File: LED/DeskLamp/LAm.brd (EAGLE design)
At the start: 34.3 x 27.3 mm, 19 parts, among them IC1 INA168, IC3 LD2985BM50R, U1 TSV621ILT

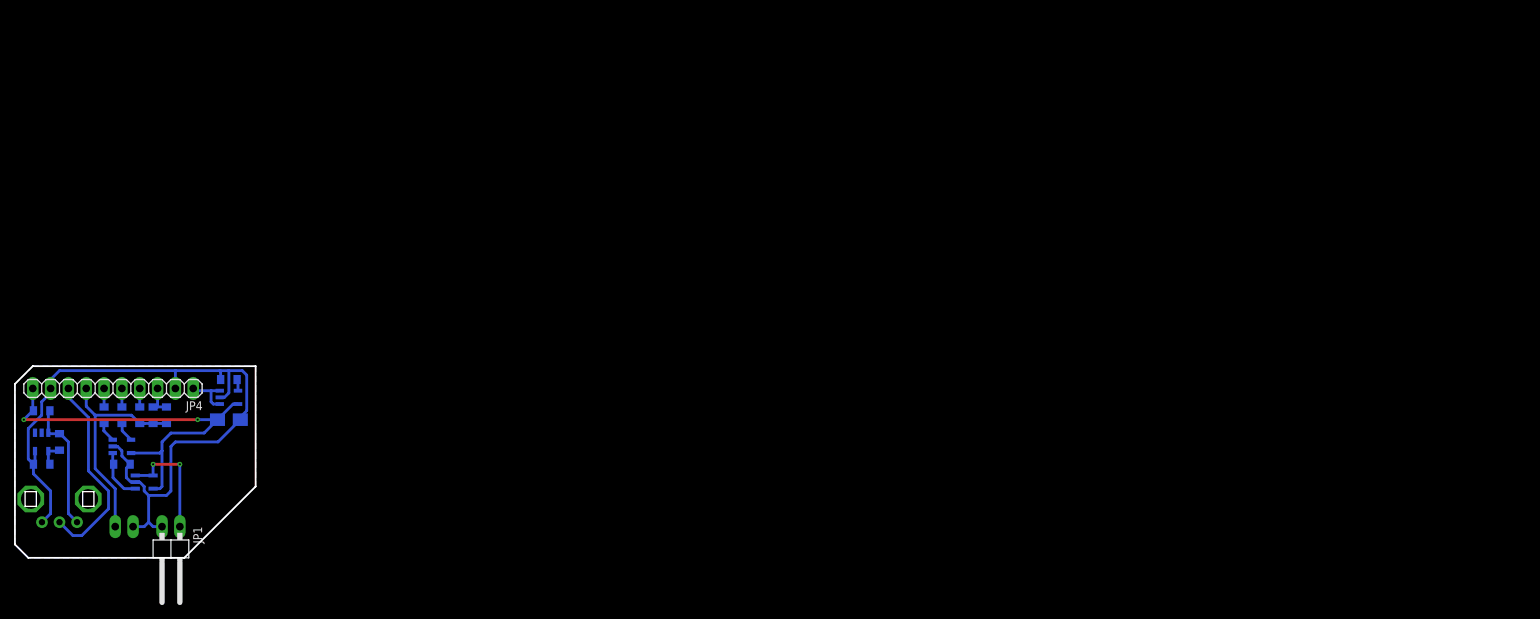
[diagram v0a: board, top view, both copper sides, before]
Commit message: DeskLamp
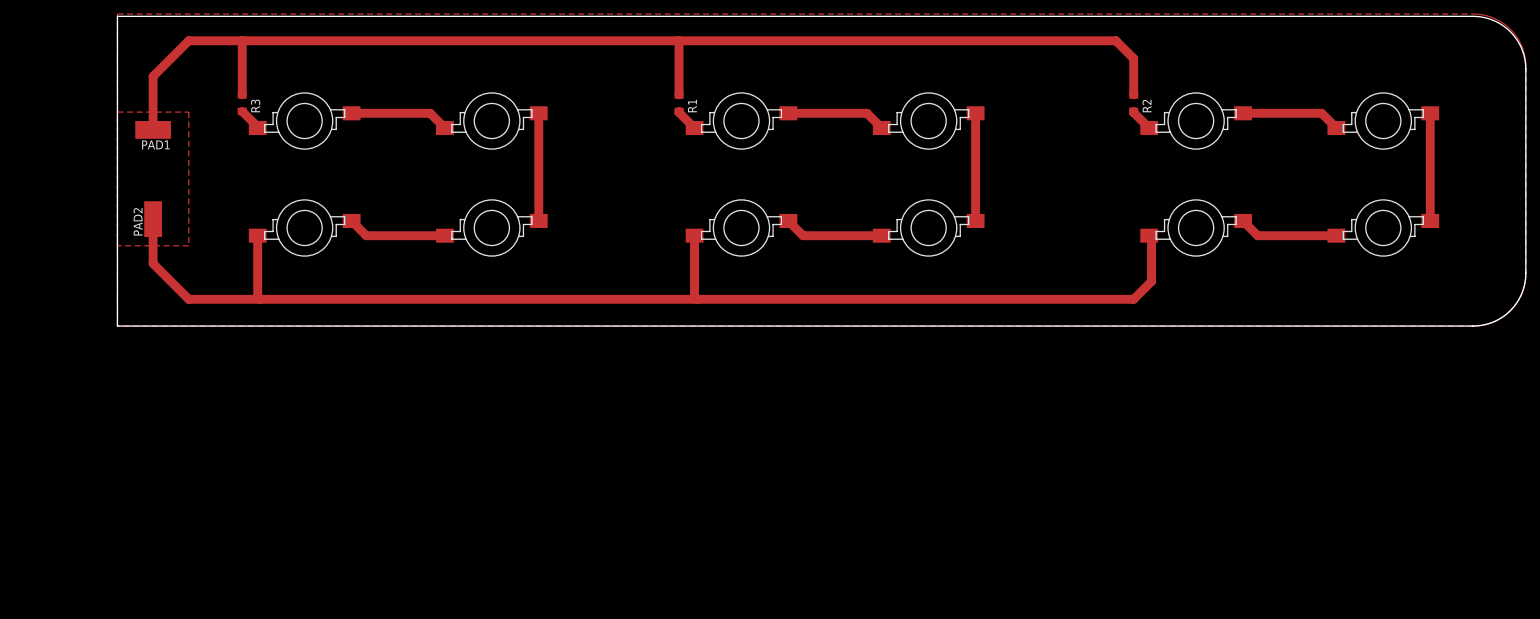
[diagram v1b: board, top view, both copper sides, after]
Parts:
- removed C1: 10n, rcl:C0805
- removed C2: 22u 16V, rcl:B/3528-21W
- removed IC1: INA168, burr-brown:SOT23-5
- removed IC3: LD2985BM50R, v-reg:SOT25
- removed JP1, JP2: (no value), pinhead:1X02/90
- removed JP4: (no value), pinhead:1X10
- removed R11, R16: 0, rcl:R0805
- removed R15: 33K, rcl:R0805
- removed R4, R6: 1K, rcl:R0805
- removed R5: 3K3, rcl:R0805
- removed R7: EVUE20, pot:EVUE
- removed U1: TSV621ILT, ST Microelctronics_By_element14_Batch_1:SOT95P280X145-5N
- added PAD1: +12, wirepad:SMD2,54-5,08
- added PAD2: 0, wirepad:SMD2,54-5,08
- added U$10, U$11, U$12, U$2, U$3, U$4, U$5, U$6, U$7, U$8, U$9: LED1W, Namenlos:LED-1W
- R1: value 9K1 -> (none)
- R2: value 820K -> (none)
- R3: value 1K -> (none)
- U$1: value TL431-IDBVR -> LED1W; device TL431:SOT23-5 -> Namenlos:LED-1W
- moved R2 144.8 mm to (144.8, 31.8), flipped to the top, turned to 270 degrees
- moved U$1 110.2 mm to (88.9, 29.2), flipped to the top, turned to 0 degrees
- moved R1 87.1 mm to (80.0, 31.8), flipped to the top, turned to 270 degrees
- moved R3 46.8 mm to (17.8, 31.8), flipped to the top
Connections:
- removed net +12V: IC3.1, IC3.3, JP4.1
- removed net +5V: C2.+, IC1.5, IC3.5, JP4.10, R4.2, U1.5
- removed net +V-FB: JP2.1, JP4.7, R1.1, R2.1, R3.2
- removed net -V-FB: JP4.8, R7.2
- removed net C-IN+: JP4.6, R11.1
- removed net C-IN-: JP4.5, R16.1
- removed net GND: C1.2, C2.-, IC1.2, IC3.2, JP1.2, JP2.2, JP4.2, JP4.9, R15.1, R5.1, R7.3, U$1.A, U1.2
- removed net V-IN+: JP4.3, R1.2, R2.2
- removed net V-IN-: JP4.4, R3.1
- new net N$10: U$10.A, U$9.K
- new net N$11: U$10.K, U$11.A
- new net N$12: U$11.K, U$12.A
- new net N$13: PAD1.1, R1.1, R2.1, R3.1
- new net N$14: PAD2.1, U$12.K, U$4.K, U$8.K
- new net N$6: U$5.K, U$6.A
- new net N$9: R3.2, U$9.A
- net N$1: now also R1.2, U$1.A; no longer R4.1, R6.2, R7.1, U$1.C
- net N$2: now also U$1.K, U$2.A; no longer R5.2, R6.1, U$1.R
- net N$3: now also U$2.K, U$3.A; no longer IC1.4, R16.2
- net N$4: now also U$3.K, U$4.A; no longer IC1.3, R11.2
- net N$5: now also R2.2, U$5.A; no longer C1.1, IC3.4
- net N$7: now also U$6.K, U$7.A; no longer JP1.1, U1.3, U1.4
- net N$8: now also U$7.K, U$8.A; no longer IC1.1, R15.2, U1.1
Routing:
- net N$14: track 0.00 -> 176.9 mm
- net N$13: track 0.00 -> 171.1 mm
- net GND: track 110.5 -> 0.00 mm
- net +5V: track 58.0 -> 0.00 mm, vias 2 -> 0
- net +V-FB: track 32.2 -> 0.00 mm
- net -V-FB: track 28.9 -> 0.00 mm
- net N$11: track 0.00 -> 15.3 mm
- net N$1: track 18.6 -> 3.28 mm
- net N$6: track 0.00 -> 14.2 mm
- net N$12: track 0.00 -> 14.2 mm
- net N$10: track 0.00 -> 14.2 mm
- net N$3: track 2.86 -> 15.3 mm
- net N$4: track 2.86 -> 14.2 mm
- net N$2: track 3.61 -> 14.2 mm
- net +12V: track 6.87 -> 0.00 mm
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- added copper zone on layer 1, net N$15
- added copper zone on layer 1, net N$16
- removed copper zone on layer 16, net GND
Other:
- board size 34.3 x 27.3 mm -> 200.6 x 44.1 mm
